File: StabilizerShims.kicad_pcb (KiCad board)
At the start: 2 copper layers, 105 x 103 mm, 42 parts

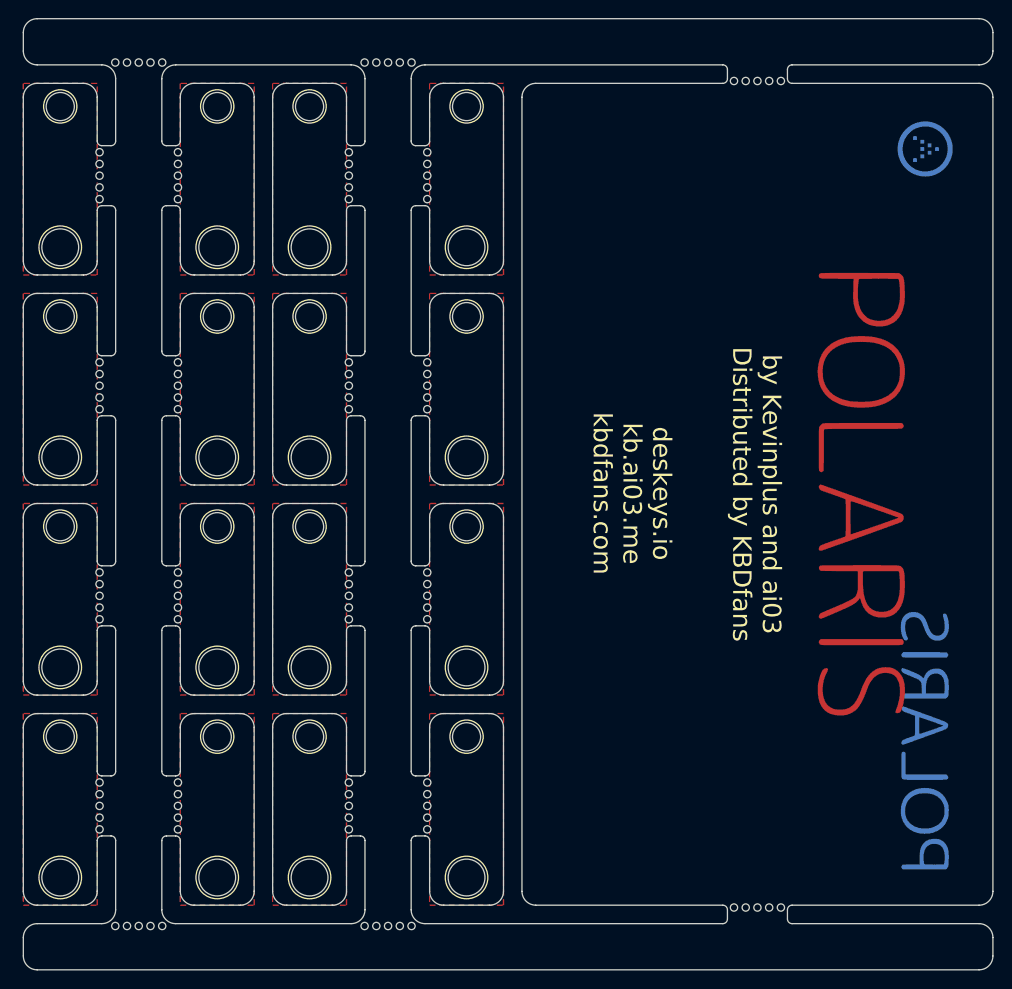
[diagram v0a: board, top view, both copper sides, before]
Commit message: V2
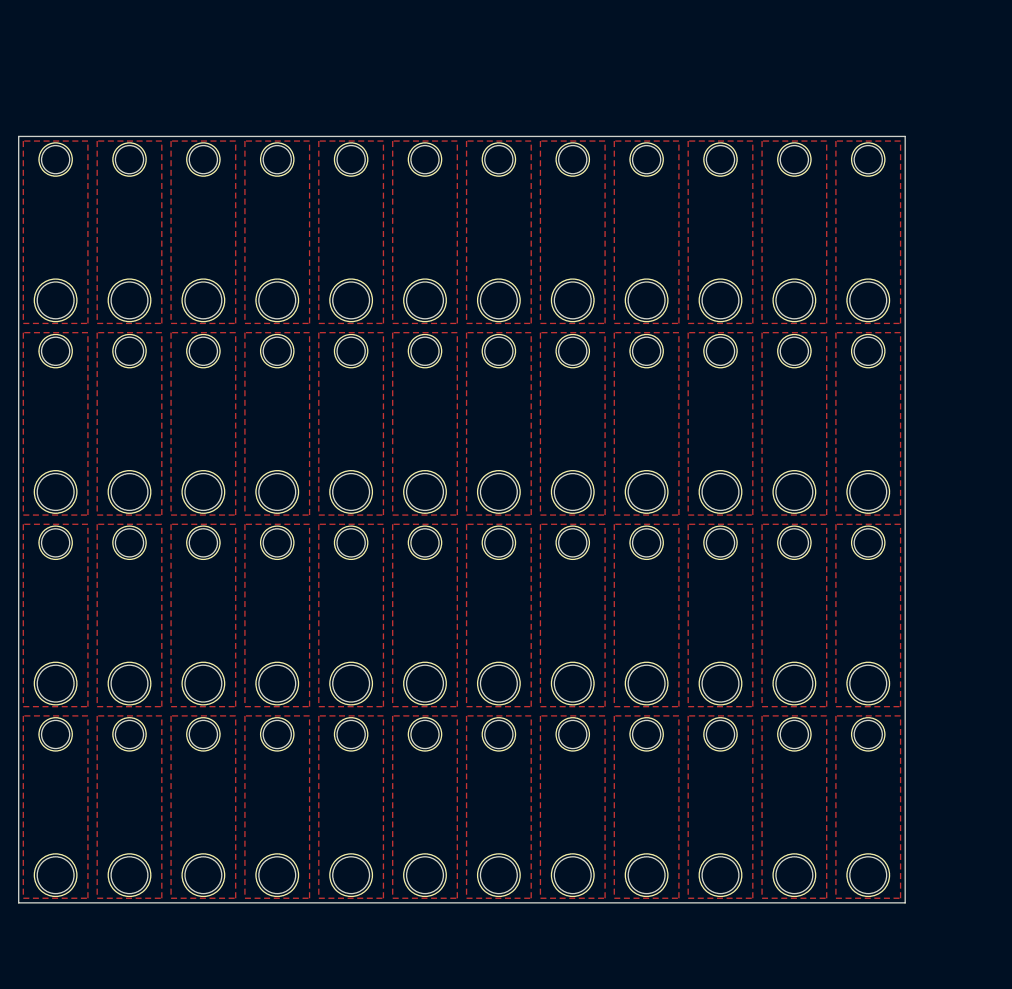
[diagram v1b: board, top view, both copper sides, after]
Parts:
- removed G***: LOGO, locallib:ai-ring-6mm-FancyAss-Mask
- removed G***: LOGO, locallib:ai-ring-6mm-FancyAss
- removed G***: LOGO, locallib:PolarisSmall
- removed G***: LOGO, locallib:PolarisLogo
- removed the REF** at (202.5, 138.2)
- removed the REF** at (154.0, 81.5)
- removed the REF** at (167.0, 82.0)
- removed the REF** at (171.0, 104.2)
- removed the REF** at (158.0, 82.0)
- removed the REF** at (158.0, 59.2)
- removed the REF** at (154.0, 58.8)
- removed the REF** at (158.0, 127.5)
- removed the REF** at (171.0, 81.5)
- removed the REF** at (171.0, 58.8)
- removed the REF** at (167.0, 127.5)
- removed the REF** at (202.5, 49.2)
- removed the REF** at (158.0, 104.8)
- removed the REF** at (154.0, 104.2)
- removed the REF** at (154.0, 127.0)
- removed the REF** at (144.0, 81.5)
- removed the REF** at (140.0, 82.0)
- removed the REF** at (140.0, 59.2)
- removed the REF** at (144.0, 58.8)
- removed the REF** at (140.0, 127.5)
- removed the REF** at (140.0, 104.8)
- removed the REF** at (144.0, 104.2)
- removed the REF** at (135.5, 140.2)
- removed the REF** at (144.0, 127.0)
- removed the REF** at (131.0, 82.0)
- removed the REF** at (131.0, 59.2)
- removed the REF** at (127.0, 58.8)
- removed the REF** at (127.0, 81.5)
- removed the REF** at (131.0, 104.8)
- removed the REF** at (127.0, 104.2)
- removed the REF** at (131.0, 127.5)
- removed the REF** at (162.5, 140.2)
- removed the REF** at (135.5, 47.2)
- removed the REF** at (162.5, 47.2)
- removed the REF** at (167.0, 59.2)
- removed the REF** at (167.0, 104.8)
- removed the REF** at (171.0, 127.0)
- added REF**: StabilizerShim-Holes, locallib:StabilizerShim-Holes, F.Cu at (214.5, 85.2)
- added REF**: StabilizerShim-Holes, locallib:StabilizerShim-Holes, F.Cu at (198.5, 64.5)
- added REF**: StabilizerShim-Holes, locallib:StabilizerShim-Holes, F.Cu at (198.5, 106.0)
- added REF**: StabilizerShim-Holes, locallib:StabilizerShim-Holes, F.Cu at (198.5, 126.8)
- added REF**: StabilizerShim-Holes, locallib:StabilizerShim-Holes, F.Cu at (190.5, 85.2)
- added REF**: StabilizerShim-Holes, locallib:StabilizerShim-Holes, F.Cu at (190.5, 64.5)
- added REF**: StabilizerShim-Holes, locallib:StabilizerShim-Holes, F.Cu at (190.5, 106.0)
- added REF**: StabilizerShim-Holes, locallib:StabilizerShim-Holes, F.Cu at (190.5, 126.8)
- added REF**: StabilizerShim-Holes, locallib:StabilizerShim-Holes, F.Cu at (182.5, 85.2)
- added REF**: StabilizerShim-Holes, locallib:StabilizerShim-Holes, F.Cu at (182.5, 64.5)
- added REF**: StabilizerShim-Holes, locallib:StabilizerShim-Holes, F.Cu at (182.5, 106.0)
- added REF**: StabilizerShim-Holes, locallib:StabilizerShim-Holes, F.Cu at (214.5, 64.5)
- added REF**: StabilizerShim-Holes, locallib:StabilizerShim-Holes, F.Cu at (182.5, 126.8)
- added REF**: StabilizerShim-Holes, locallib:StabilizerShim-Holes, F.Cu at (174.5, 85.2)
- added REF**: StabilizerShim-Holes, locallib:StabilizerShim-Holes, F.Cu at (174.5, 64.5)
- added REF**: StabilizerShim-Holes, locallib:StabilizerShim-Holes, F.Cu at (174.5, 106.0)
- added REF**: StabilizerShim-Holes, locallib:StabilizerShim-Holes, F.Cu at (174.5, 126.8)
- added REF**: StabilizerShim-Holes, locallib:StabilizerShim-Holes, F.Cu at (166.5, 85.2)
- added REF**: StabilizerShim-Holes, locallib:StabilizerShim-Holes, F.Cu at (166.5, 64.5)
- added REF**: StabilizerShim-Holes, locallib:StabilizerShim-Holes, F.Cu at (166.5, 106.0)
- added REF**: StabilizerShim-Holes, locallib:StabilizerShim-Holes, F.Cu at (166.5, 126.8)
- added REF**: StabilizerShim-Holes, locallib:StabilizerShim-Holes, F.Cu at (158.5, 85.2)
- added REF**: StabilizerShim-Holes, locallib:StabilizerShim-Holes, F.Cu at (214.5, 106.0)
- added REF**: StabilizerShim-Holes, locallib:StabilizerShim-Holes, F.Cu at (158.5, 64.5)
- added REF**: StabilizerShim-Holes, locallib:StabilizerShim-Holes, F.Cu at (158.5, 106.0)
- added REF**: StabilizerShim-Holes, locallib:StabilizerShim-Holes, F.Cu at (158.5, 126.8)
- added REF**: StabilizerShim-Holes, locallib:StabilizerShim-Holes, F.Cu at (150.5, 85.2)
- added REF**: StabilizerShim-Holes, locallib:StabilizerShim-Holes, F.Cu at (150.5, 64.5)
- added REF**: StabilizerShim-Holes, locallib:StabilizerShim-Holes, F.Cu at (150.5, 106.0)
- added REF**: StabilizerShim-Holes, locallib:StabilizerShim-Holes, F.Cu at (150.5, 126.8)
- added REF**: StabilizerShim-Holes, locallib:StabilizerShim-Holes, F.Cu at (142.5, 85.2)
- added REF**: StabilizerShim-Holes, locallib:StabilizerShim-Holes, F.Cu at (142.5, 64.5)
- added REF**: StabilizerShim-Holes, locallib:StabilizerShim-Holes, F.Cu at (142.5, 106.0)
- added REF**: StabilizerShim-Holes, locallib:StabilizerShim-Holes, F.Cu at (214.5, 126.8)
- added REF**: StabilizerShim-Holes, locallib:StabilizerShim-Holes, F.Cu at (142.5, 126.8)
- added REF**: StabilizerShim-Holes, locallib:StabilizerShim-Holes, F.Cu at (134.5, 85.2)
- added REF**: StabilizerShim-Holes, locallib:StabilizerShim-Holes, F.Cu at (134.5, 64.5)
- added REF**: StabilizerShim-Holes, locallib:StabilizerShim-Holes, F.Cu at (134.5, 106.0)
- added REF**: StabilizerShim-Holes, locallib:StabilizerShim-Holes, F.Cu at (134.5, 126.8)
- added REF**: StabilizerShim-Holes, locallib:StabilizerShim-Holes, F.Cu at (126.5, 64.5)
- added REF**: StabilizerShim-Holes, locallib:StabilizerShim-Holes, F.Cu at (126.5, 85.2)
- added REF**: StabilizerShim-Holes, locallib:StabilizerShim-Holes, F.Cu at (126.5, 106.0)
- added REF**: StabilizerShim-Holes, locallib:StabilizerShim-Holes, F.Cu at (206.5, 85.2)
- added REF**: StabilizerShim-Holes, locallib:StabilizerShim-Holes, F.Cu at (206.5, 64.5)
- added REF**: StabilizerShim-Holes, locallib:StabilizerShim-Holes, F.Cu at (206.5, 106.0)
- added REF**: StabilizerShim-Holes, locallib:StabilizerShim-Holes, F.Cu at (206.5, 126.8)
- added REF**: StabilizerShim-Holes, locallib:StabilizerShim-Holes, F.Cu at (198.5, 85.2)
- moved REF** 0.56 mm to (126.5, 126.8)
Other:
- board size 105 x 103 mm -> 96 x 83 mm
- board text added: "V-CUT"
- board text removed: "Assembled by"
- board text removed: "Plate:"
- board text removed: "Stabilizers:"
- board text removed: "Switches:"
- board text removed: "by Kevinplus and ai03 Distributed by KBDfans"
- board text removed: "deskeys.io kb.ai03.me kbdfans.com"
